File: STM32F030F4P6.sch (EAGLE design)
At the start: 28 parts, among them IC1 MCP170333MB, J3 455-1750-1-ND, J4 CORTEX_DEBUG_MINIMUM_PTH, U1 STM32F030F4P6

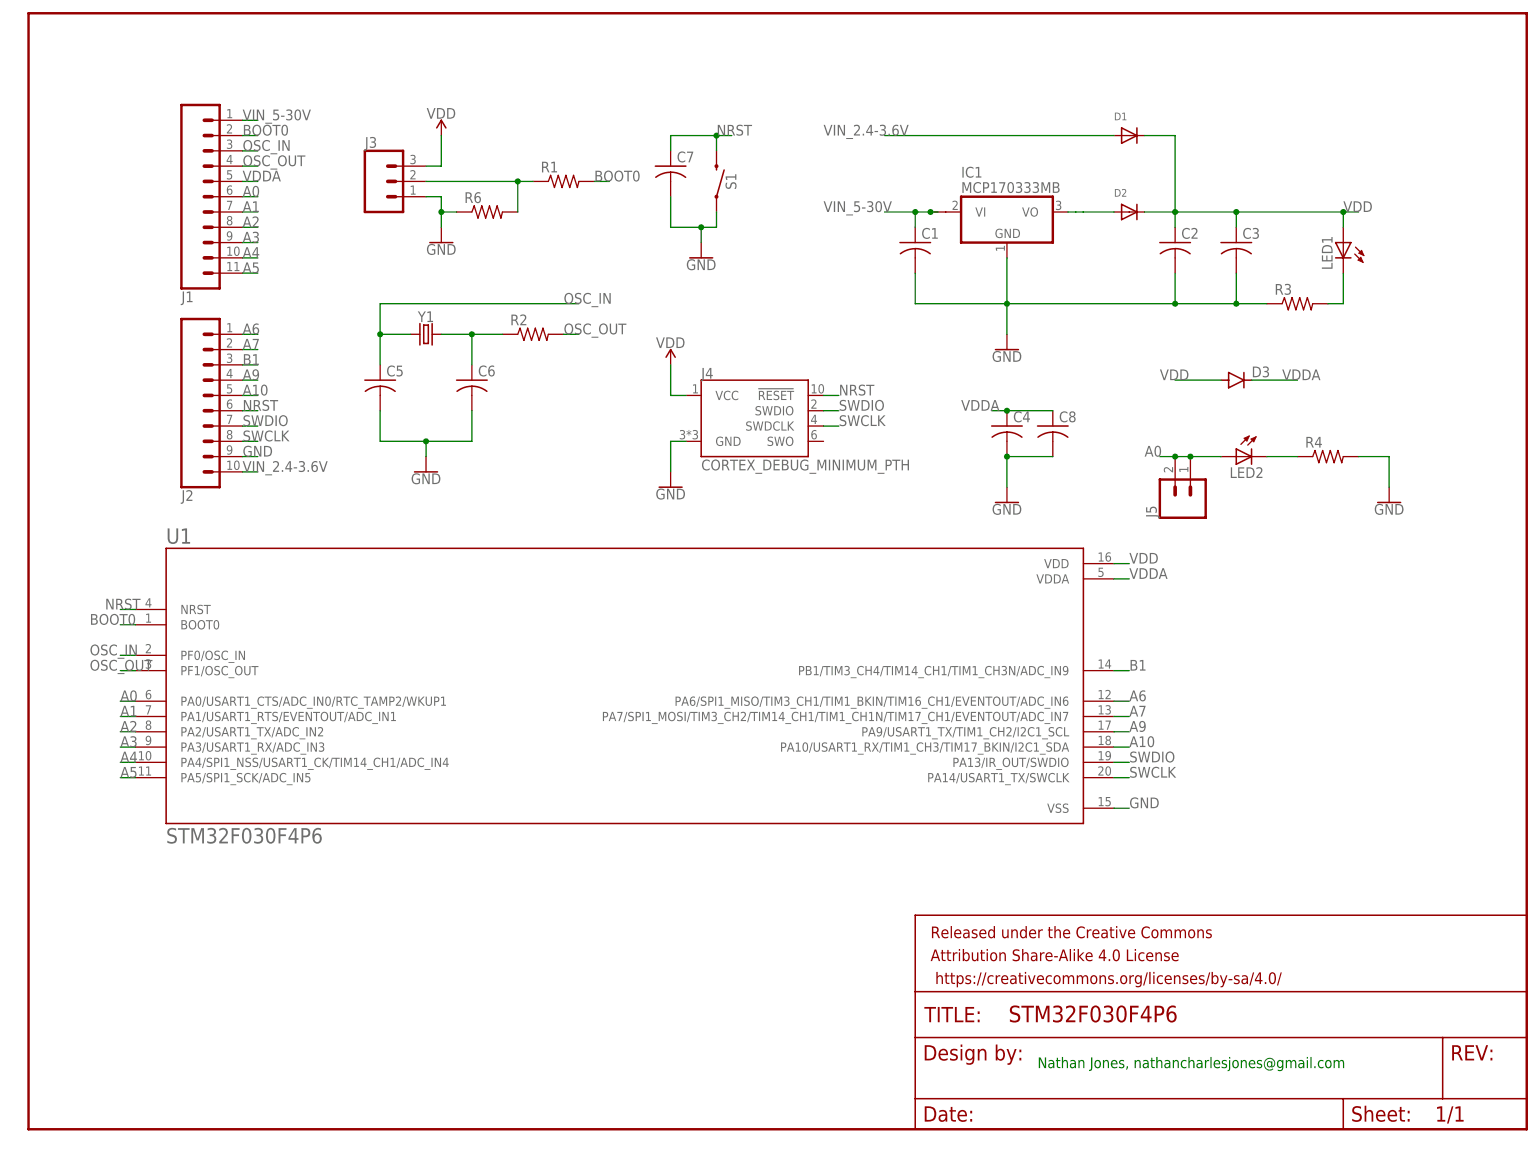
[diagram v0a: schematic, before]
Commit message: Finished.
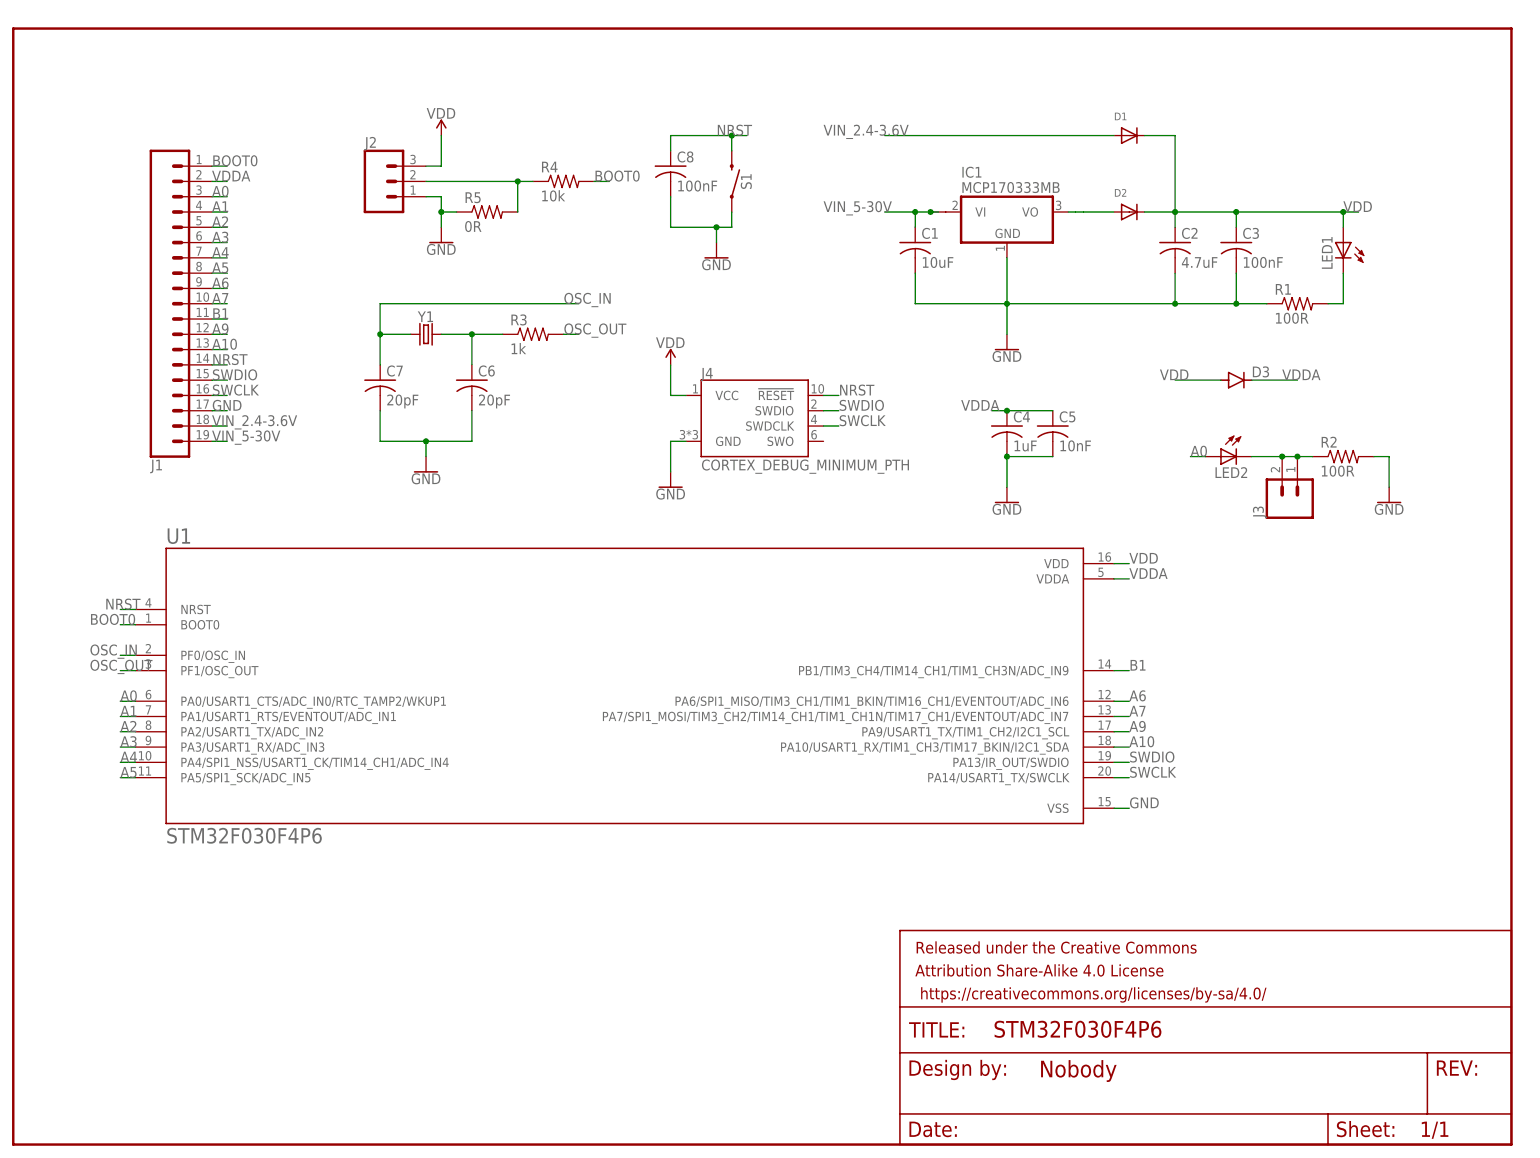
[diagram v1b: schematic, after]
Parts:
- removed FRAME1: FRAME-LETTER, SparkFun-Aesthetics:FRAME-LETTER
- removed J5: (no value), SparkFun-Connectors:CONN_02
- added FRAME2: FRAME-LETTERNO_PACKAGE, SparkFun-Aesthetics:FRAME-LETTERNO_PACKAGE
- C1: value (none) -> 10uF
- C2: value (none) -> 4.7uF
- C3, C8: value (none) -> 100nF
- C4: value (none) -> 1uF
- C5: value (none) -> 10nF
- C6, C7: value (none) -> 20pF
- J1: device SparkFun-Connectors:CONN_11 -> SparkFun-Connectors:CONN_19
- J2: value (none) -> 455-1750-1-ND; device SparkFun-Connectors:CONN_10" -> SparkFun-Connectors:CONN_03
- J3: value 455-1750-1-ND -> (none); device SparkFun-Connectors:CONN_03 -> SparkFun-Connectors:CONN_02
- R1, R2: value (none) -> 100R
- R3: value (none) -> 1k
- R4: value (none) -> 10k
- R5: value (none) -> 0R
- renumbered R6 to R5
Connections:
- removed net N$8: LED2.C, R4.1
- new net N$2: J3.1, J3.2, LED2.C, R2.1
- net A0: now also J1.3; no longer J1.6, J5.1, J5.2
- net A1: now also J1.4; no longer J1.7
- net A10: now also J1.13; no longer J2.5
- net A2: now also J1.5; no longer J1.8
- net A3: now also J1.6; no longer J1.9
- net A4: now also J1.7; no longer J1.10
- net A5: now also J1.8; no longer J1.11
- net A6: now also J1.9; no longer J2.1
- net A7: now also J1.10; no longer J2.2
- net A9: now also J1.12; no longer J2.4
- net B1: now also J1.11; no longer J2.3
- net BOOT0: now also J1.1, R4.2; no longer J1.2, R1.2
- net GND: now also J1.17, J2.1, R1.1, R2.2; no longer J2.9, J3.1, R3.1, R4.2
- net N$1: now also J2.2, R4.1; no longer J3.2, R1.1
- net N$3: now also R3.1; no longer R2.1
- net N$7: now also R1.2; no longer R3.2
- net NRST: now also C8.1, J1.14; no longer C7.1, J2.6
- net OSC_IN: now also C7.1; no longer C5.1, J1.3
- net OSC_OUT: now also R3.2; no longer J1.4, R2.2
- net SWCLK: now also J1.16; no longer J2.8
- net SWDIO: now also J1.15; no longer J2.7
- net VDD: now also J2.3; no longer J3.3
- net VDDA: now also C5.1, J1.2; no longer C8.1, J1.5
- net VIN_2.4-3.6V: now also J1.18; no longer J2.10
- net VIN_5-30V: now also J1.19; no longer J1.1
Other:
- note removed: "Nathan Jones, nathancharlesjones@gmail.com"
- moved on the sheet: C5, C7, C8, LED2, R1, R2, R3, R4, S1
